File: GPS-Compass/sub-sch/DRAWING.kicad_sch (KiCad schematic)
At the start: 0 parts

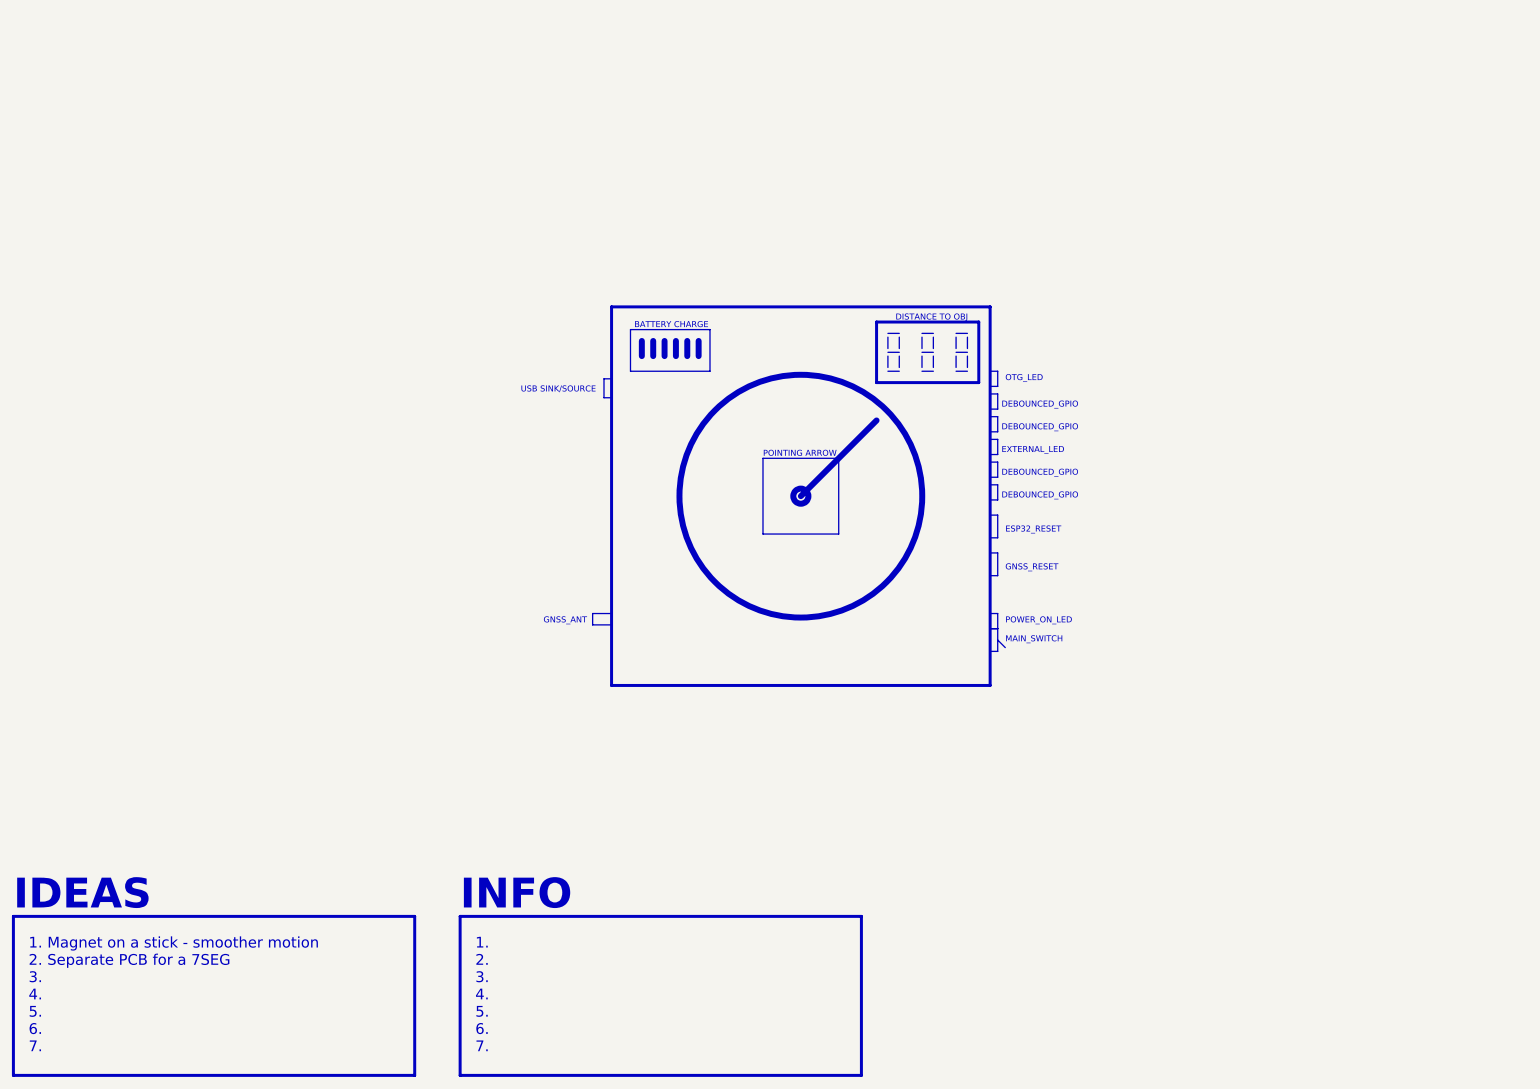
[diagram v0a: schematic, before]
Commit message: sdas
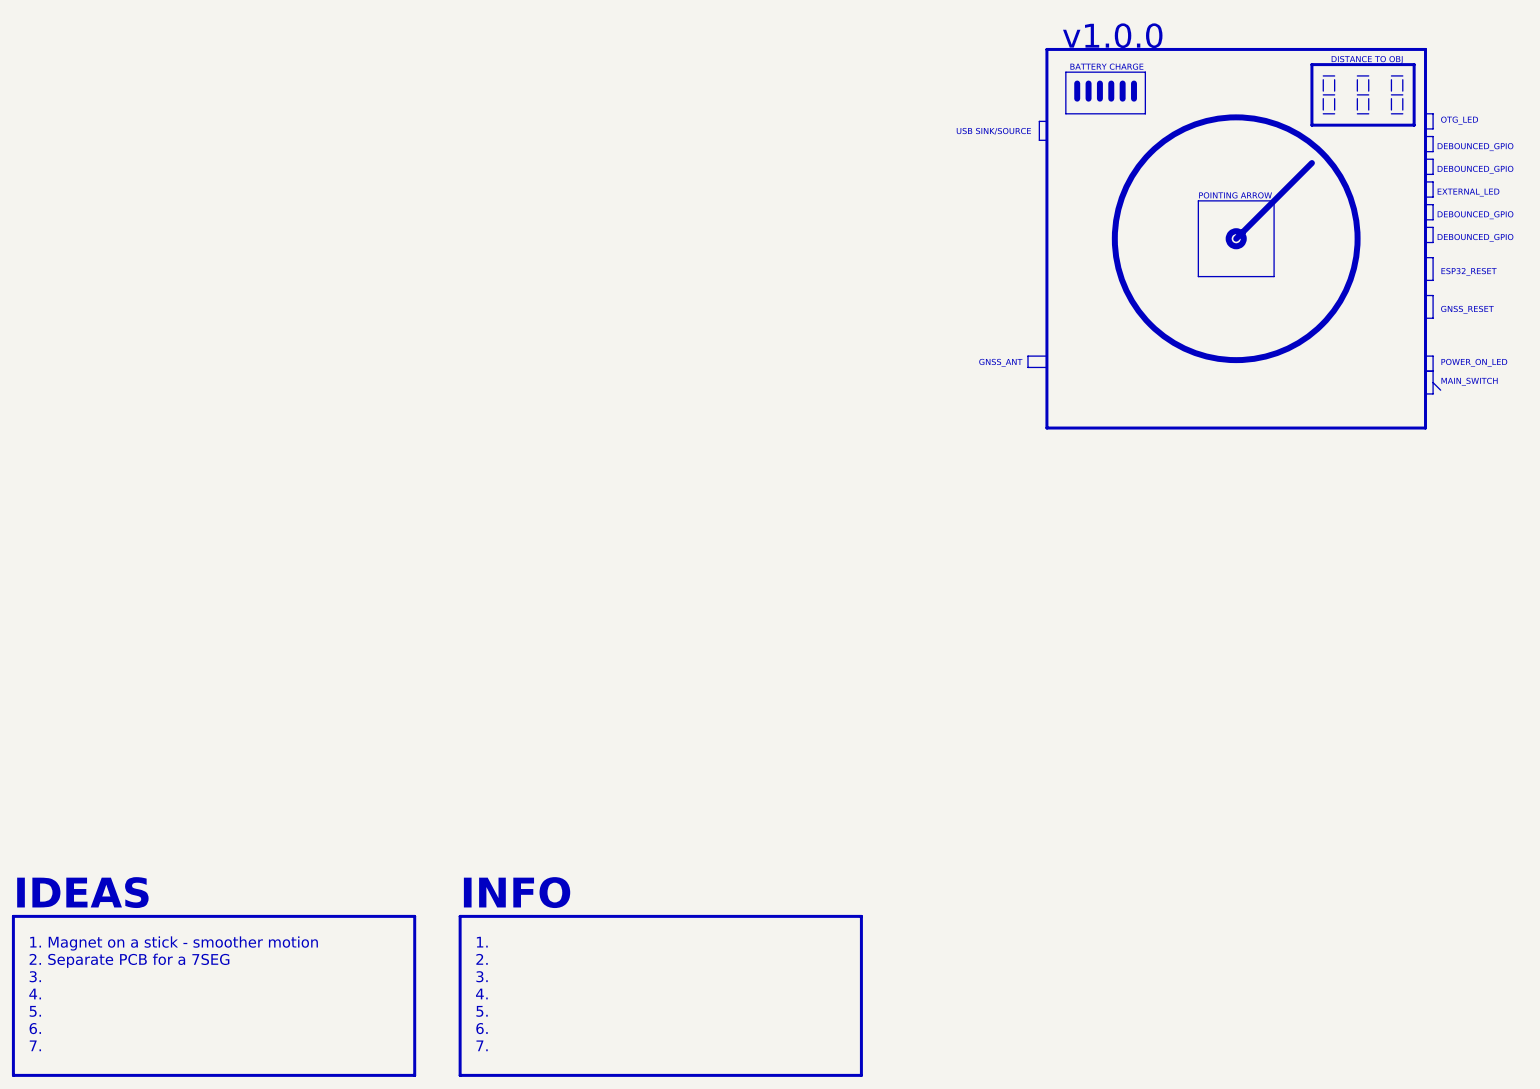
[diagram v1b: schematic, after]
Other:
- note added: "v1.0.0"
